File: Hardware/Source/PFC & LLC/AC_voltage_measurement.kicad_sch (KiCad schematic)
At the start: 17 parts, among them U5 OP07CSZ, U6 MCP1525T-I/TT

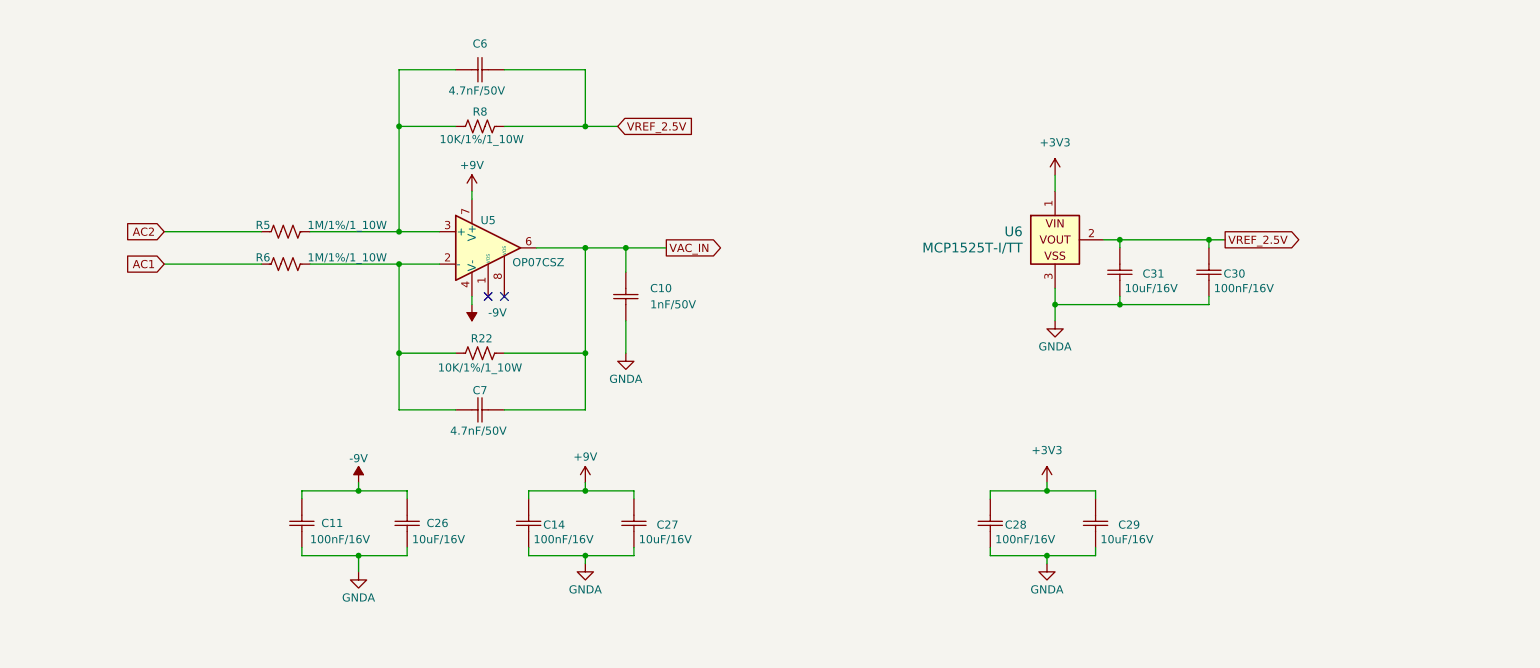
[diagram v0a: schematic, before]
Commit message: update FEEDBACK, AC
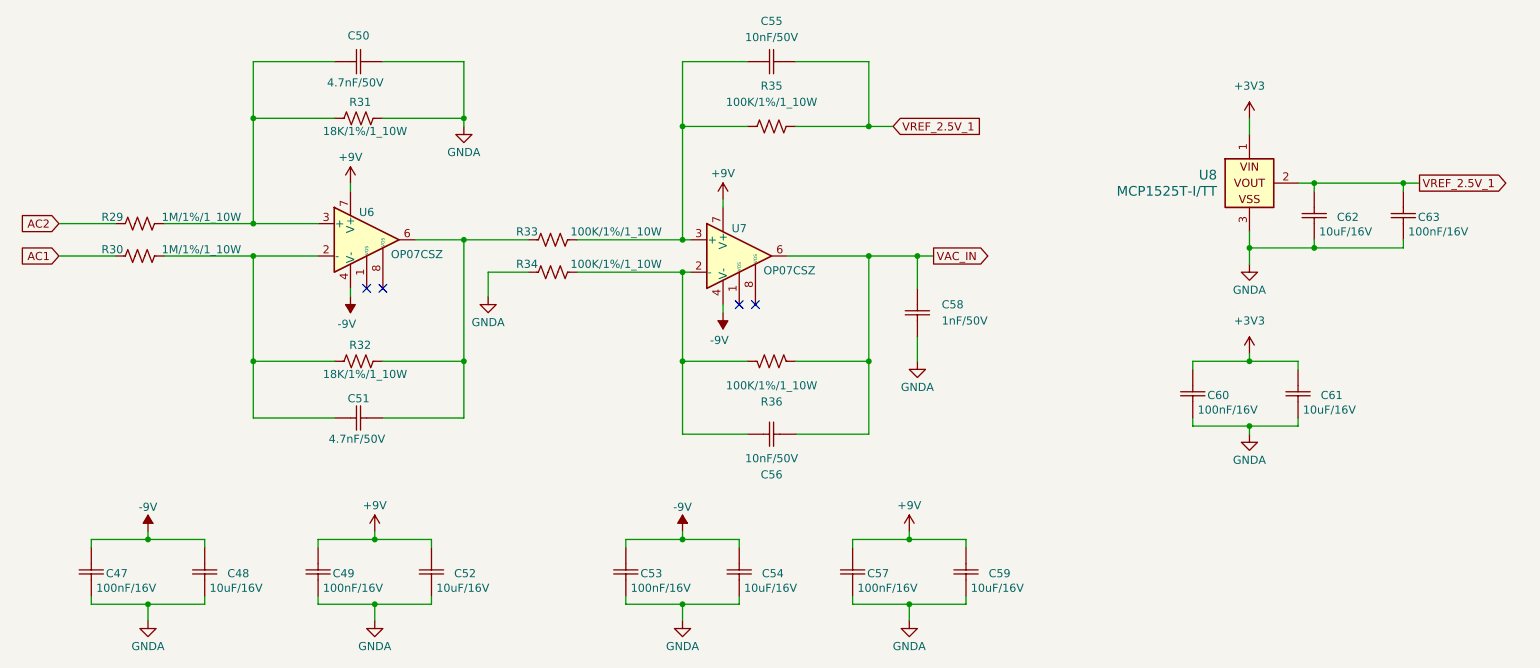
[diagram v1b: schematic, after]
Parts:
- removed C10: 1nF/50V, charge_battery_footprint_lib:Ceramic_Cap_0603, symbol charge_battery_sym_lib:Ceramic_Cap_SMD_1nF_50V
- removed C11: 100nF/16V, charge_battery_footprint_lib:Ceramic_Cap_0603, symbol charge_battery_sym_lib:Ceramic_Cap_SMD_100nF_16V
- removed C26: 10uF/16V, charge_battery_footprint_lib:Ceramic_Cap_0603, symbol charge_battery_sym_lib:Ceramic_Cap_SMD_10uF_16V
- removed R22, R8: 10K/1%/1_10W, charge_battery_footprint_lib:Res_0603, symbol charge_battery_sym_lib:Res_10K_0603_1%
- removed R6: 1M/1%/1_10W, charge_battery_footprint_lib:Res_0603, symbol charge_battery_sym_lib:Res_1M_0603_1%
- added C47, C53, C57: 100nF/16V, charge_battery_footprint_lib:Ceramic_Cap_0603, symbol charge_battery_sym_lib:Ceramic_Cap_SMD_100nF_16V
- added C48, C54, C59: 10uF/16V, charge_battery_footprint_lib:Ceramic_Cap_0603, symbol charge_battery_sym_lib:Ceramic_Cap_SMD_10uF_16V
- added C55, C56: 10nF/50V, charge_battery_footprint_lib:Ceramic_Cap_0603, symbol charge_battery_sym_lib:Ceramic_Cap_SMD_10nF_50V
- added C58: 1nF/50V, charge_battery_footprint_lib:Ceramic_Cap_0603, symbol charge_battery_sym_lib:Ceramic_Cap_SMD_1nF_50V
- added R30: 1M/1%/1_10W, charge_battery_footprint_lib:Res_0603, symbol charge_battery_sym_lib:Res_1M_0603_1%
- added R31, R32: 18K/1%/1_10W, charge_battery_footprint_lib:Res_0603, symbol charge_battery_sym_lib:Res_18K_0603_1%
- added R33, R34, R35, R36: 100K/1%/1_10W, charge_battery_footprint_lib:Res_0603, symbol charge_battery_sym_lib:Res_100K_0603_1%
- added U7: OP07CSZ, charge_battery_footprint_lib:SOIC-8, symbol charge_battery_sym_lib:OP07CSZ
- renumbered C14 to C49, C6 to C50, C7 to C51, C27 to C52, C28 to C60, C29 to C61, C31 to C62, C30 to C63, R5 to R29, U5 to U6, U6 to U8
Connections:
- net +9V: now also C57.2, C59.2, U7.7 (V+)
- net -9V: now also C47.2, C48.2, C53.2, C54.2, U7.4 (V-)
- net AC1: now also R30.1
- net GNDA: now also C50.2, C47.1, C48.1, C53.1, C54.1, C57.1, C58.1, C59.1, R31.1, R34.1
- net VAC_IN: now also C56.2, C58.2, R36.2, U7.6; no longer C51.2, U6.6
- net at C50.1, R29.2, U6.3 (+): now also R31.2
- net at C51.1, U6.2 (-): now also R30.2, R32.2
- net VREF_2.5V renamed VREF_2.5V_1
- net VREF_2.5V_1: now also C55.2, R35.2; no longer C50.2
- new net: C56.1, R34.2, R36.1, U7.2 (-)
- new net: C55.1, R33.2, R35.1, U7.3 (+)
- new net: C51.2, R32.1, R33.1, U6.6
- no-connect marks 2 -> 4
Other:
- moved on the sheet: C49, C50, C51, C52, C60, C61, C62, C63, R29, U6, U8
